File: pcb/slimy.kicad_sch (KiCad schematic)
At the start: 3 parts, among them U1 Teensy3.2, U2 PIM447

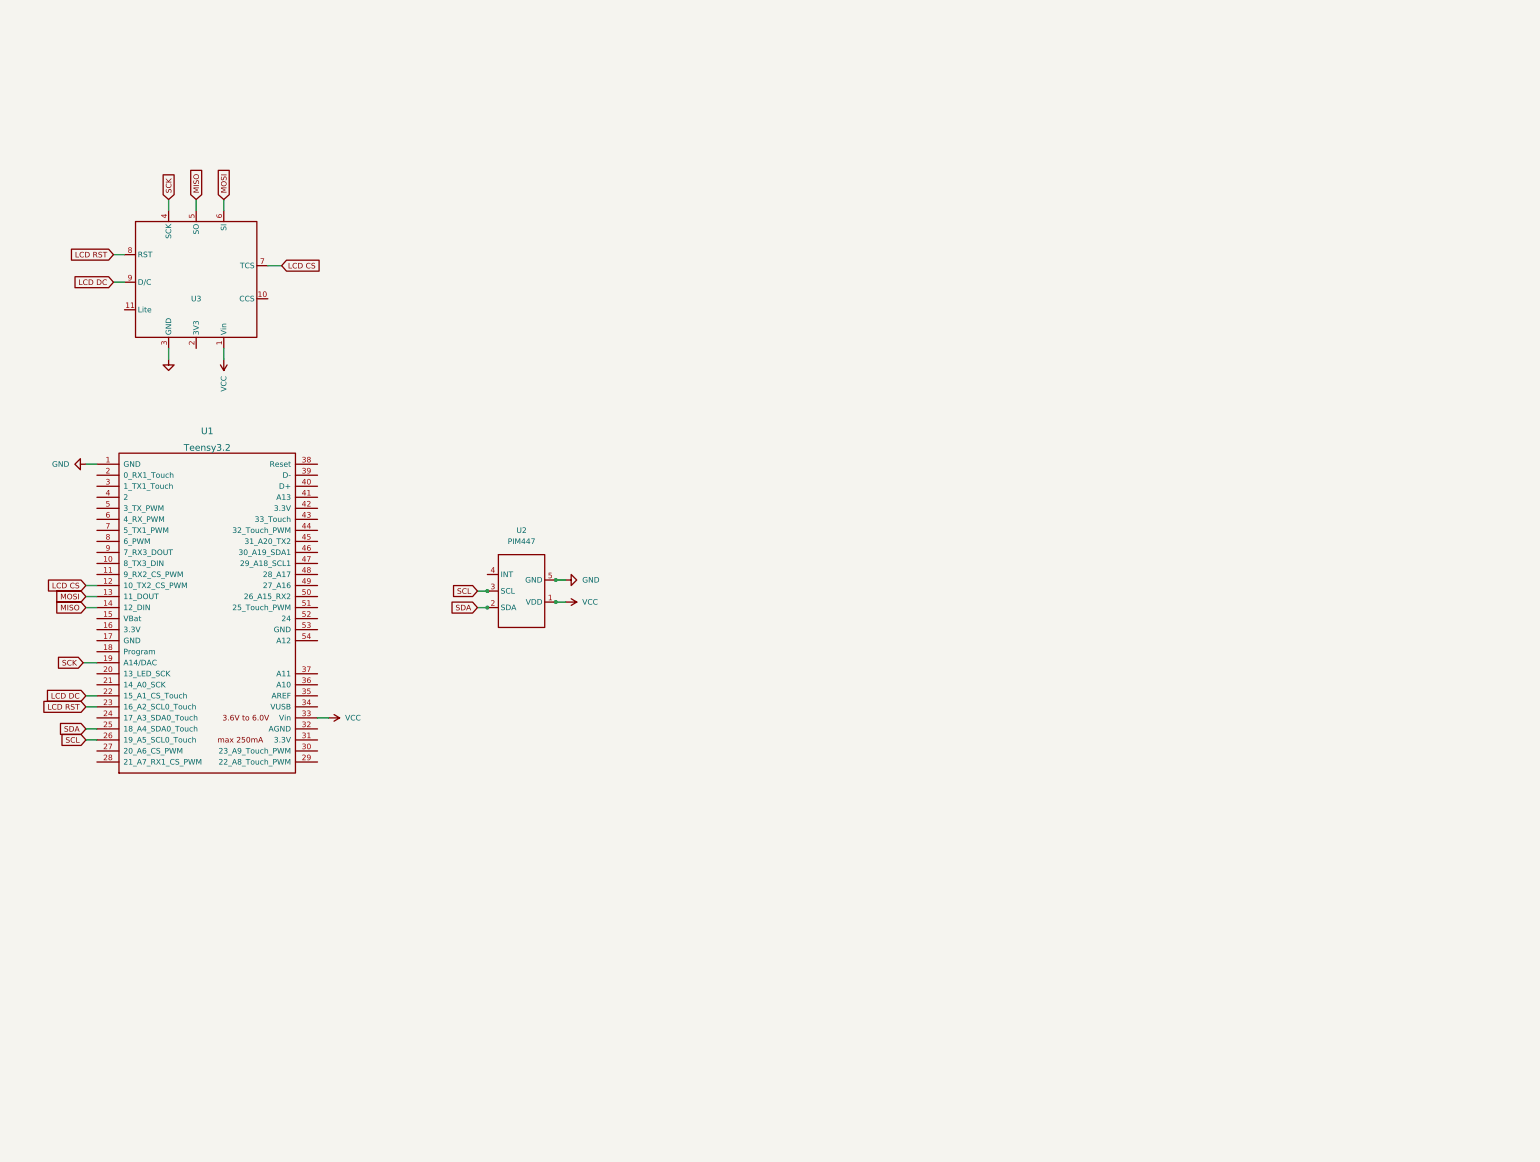
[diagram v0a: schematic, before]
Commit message: WIP keyboard pcb design
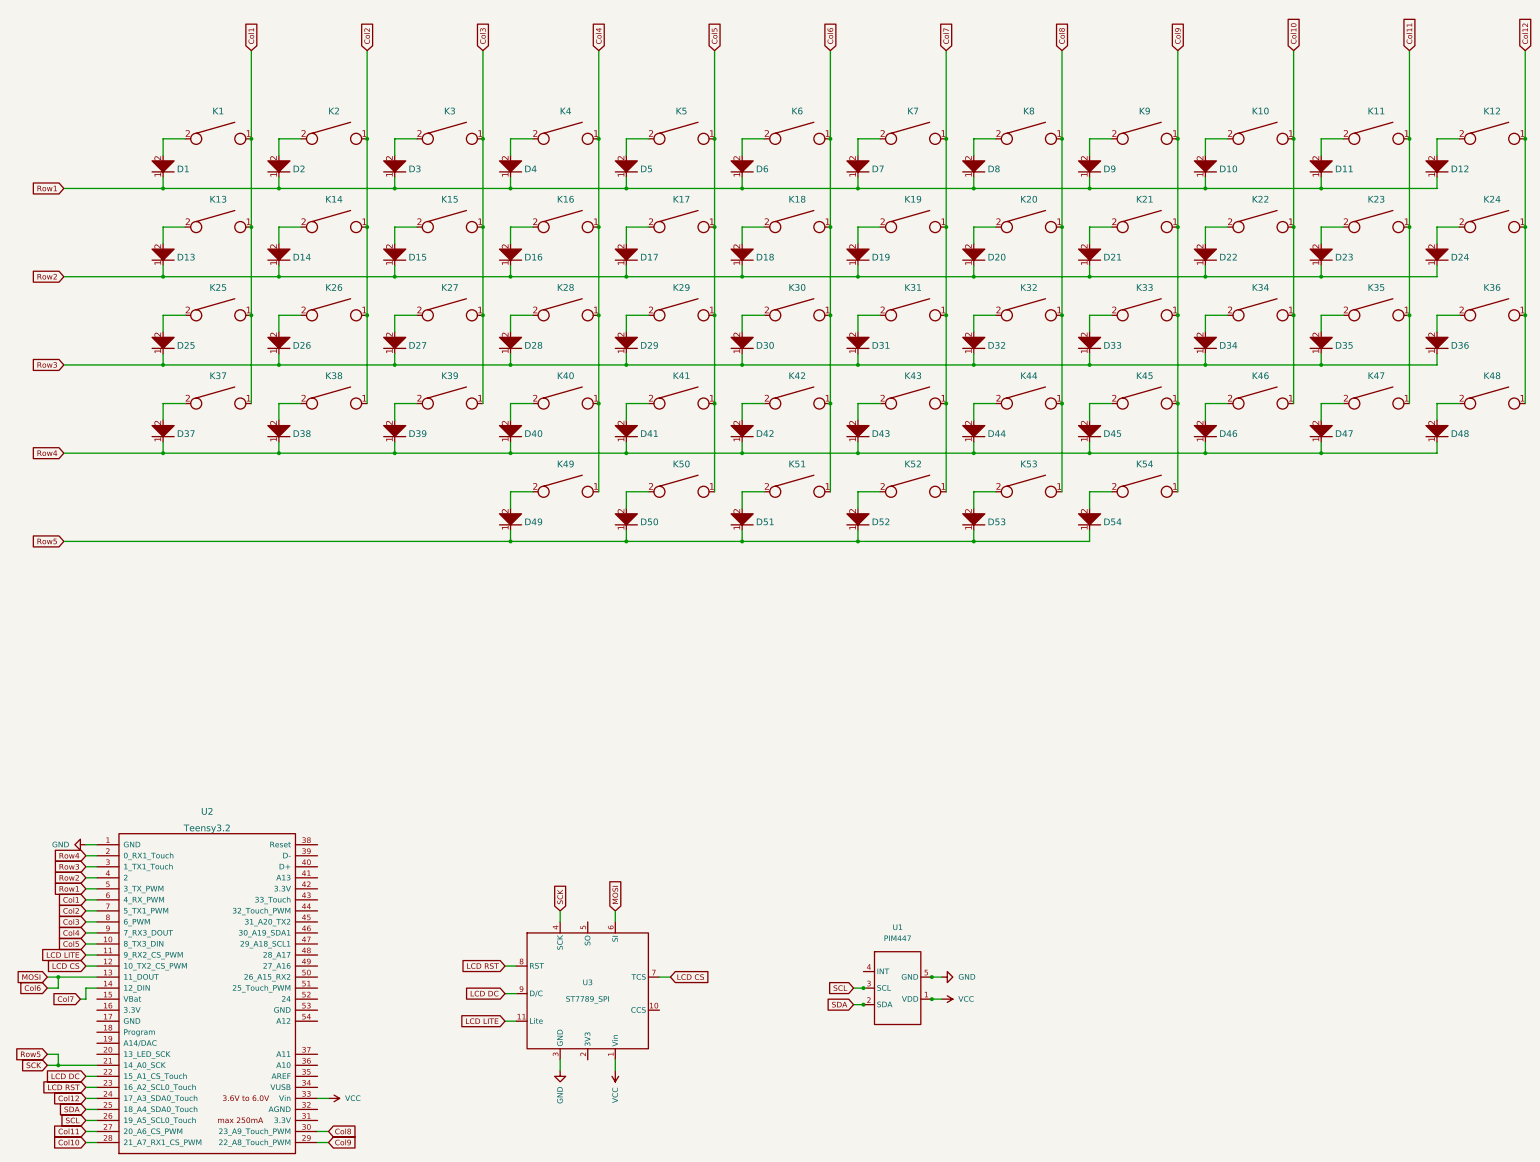
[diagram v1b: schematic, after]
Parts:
- removed U3: (no value), symbol my_lib:ST7789_240x240
- added D1, D10, D11, D12, D13, D14, D15, D16, D17, D18, D19, D2, D20, D21, D22, D23, D24, D25, D26, D27, D28, D29, D3, D30, D31, D32, D33, D34, D35, D36, D37, D38, D39, D4, D40, D41, D42, D43, D44, D45, D46, D47, D48, D49, D5, D50, D51, D52, D53, D54, D6, D7, D8, D9: D, my_lib:D_SOD123_axial, symbol kicad_lib_tmk:D
- added K1, K10, K11, K12, K13, K14, K15, K16, K17, K18, K19, K2, K20, K21, K22, K23, K24, K25, K26, K27, K28, K29, K3, K30, K31, K32, K33, K34, K35, K36, K37, K38, K39, K4, K40, K41, K42, K43, K44, K45, K46, K47, K48, K49, K5, K50, K51, K52, K53, K54, K6, K7, K8, K9: KEYSW, my_lib:MX-1U-Hotswap-Antishear, symbol kicad_lib_tmk:KEYSW
- added U3: ST7789_SPI, my_lib:ST7789_1.3_240x240, symbol my_lib:ST7789_SPI
- U1: renamed from U2; footprint (none) -> my_lib:PIM447
- U2: renamed from U1; footprint (none) -> teensy:Teensy30_31_32_All_Pins
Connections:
- net GND: now also U3.3 (GND)
- net LCD CS: now also U3.7 (TCS)
- net LCD DC: now also U3.9 (D/C)
- net LCD RST: now also U3.8 (RST)
- net VCC: now also U3.1 (Vin)
- net Col5: now reaches U2.10 (8_TX3_DIN)
- net Col5: now also K17.1, K29.1, K41.1, K5.1, K50.1
- net LCD LITE: now reaches U2.11 (9_RX2_CS_PWM)
- net LCD LITE: now also U3.11 (Lite)
- net Row4: now reaches U2.2 (0_RX1_Touch)
- net Row4: now also D37.1, D38.1, D39.1, D40.1, D41.1, D42.1, D43.1, D44.1, D45.1, D46.1, D47.1, D48.1
- net Row5: now reaches U2.21 (14_A0_SCK)
- net Row5: now also D49.1, D50.1, D51.1, D52.1, D53.1, D54.1, U3.4 (SCK)
- net Col12: now reaches U2.24 (17_A3_SDA0_Touch)
- net Col12: now also K12.1, K24.1, K36.1, K48.1
- net Col11: now reaches U2.27 (20_A6_CS_PWM)
- net Col11: now also K11.1, K23.1, K35.1, K47.1
- net Col10: now reaches U2.28 (21_A7_RX1_CS_PWM)
- net Col10: now also K10.1, K22.1, K34.1, K46.1
- net Col9: now reaches U2.29 (22_A8_Touch_PWM)
- net Col9: now also K21.1, K33.1, K45.1, K54.1, K9.1
- net Row3: now reaches U2.3 (1_TX1_Touch)
- net Row3: now also D25.1, D26.1, D27.1, D28.1, D29.1, D30.1, D31.1, D32.1, D33.1, D34.1, D35.1, D36.1
- net Col8: now reaches U2.30 (23_A9_Touch_PWM)
- net Col8: now also K20.1, K32.1, K44.1, K53.1, K8.1
- net Row2: now reaches U2.4 (2)
- net Row2: now also D13.1, D14.1, D15.1, D16.1, D17.1, D18.1, D19.1, D20.1, D21.1, D22.1, D23.1, D24.1
- net Row1: now reaches U2.5 (3_TX_PWM)
- net Row1: now also D1.1, D10.1, D11.1, D12.1, D2.1, D3.1, D4.1, D5.1, D6.1, D7.1, D8.1, D9.1
- net Col1: now reaches U2.6 (4_RX_PWM)
- net Col1: now also K1.1, K13.1, K25.1, K37.1
- net Col2: now reaches U2.7 (5_TX1_PWM)
- net Col2: now also K14.1, K2.1, K26.1, K38.1
- net Col3: now reaches U2.8 (6_PWM)
- net Col3: now also K15.1, K27.1, K3.1, K39.1
- net Col4: now reaches U2.9 (7_RX3_DOUT)
- net Col4: now also K16.1, K28.1, K4.1, K40.1, K49.1
- net MISO renamed Col7
- net Col7: now also K19.1, K31.1, K43.1, K52.1, K7.1
- net MOSI renamed Col6
- net Col6: now also K18.1, K30.1, K42.1, K51.1, K6.1, U3.6 (SI)
- net SCK: no longer names the net of U2.19 (A14/DAC)
- new net: D16.2, K16.2
- new net: D44.2, K44.2
- new net: D33.2, K33.2
- new net: D17.2, K17.2
- new net: D42.2, K42.2
- new net: D36.2, K36.2
- new net: D11.2, K11.2
- new net: D41.2, K41.2
- new net: D5.2, K5.2
- new net: D6.2, K6.2
- new net: D15.2, K15.2
- new net: D48.2, K48.2
- new net: D28.2, K28.2
- new net: D46.2, K46.2
- new net: D34.2, K34.2
- new net: D21.2, K21.2
- new net: D24.2, K24.2
- new net: D31.2, K31.2
- new net: D40.2, K40.2
- new net: D20.2, K20.2
- new net: D12.2, K12.2
- new net: D29.2, K29.2
- new net: D2.2, K2.2
- new net: D18.2, K18.2
- new net: D4.2, K4.2
- new net: D49.2, K49.2
- new net: D43.2, K43.2
- new net: D37.2, K37.2
- new net: D7.2, K7.2
- new net: D8.2, K8.2
- new net: D9.2, K9.2
- new net: D10.2, K10.2
- new net: D54.2, K54.2
- new net: D32.2, K32.2
- new net: D52.2, K52.2
- new net: D38.2, K38.2
- new net: D13.2, K13.2
- new net: D25.2, K25.2
- new net: D53.2, K53.2
- new net: D22.2, K22.2
- new net: D26.2, K26.2
- new net: D23.2, K23.2
- new net: D50.2, K50.2
- new net: D30.2, K30.2
- new net: D27.2, K27.2
- new net: D19.2, K19.2
- new net: D1.2, K1.2
- new net: D14.2, K14.2
- new net: D39.2, K39.2
- new net: D35.2, K35.2
- new net: D45.2, K45.2
- new net: D3.2, K3.2
- new net: D47.2, K47.2
- new net: D51.2, K51.2
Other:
- moved on the sheet: U1, U2

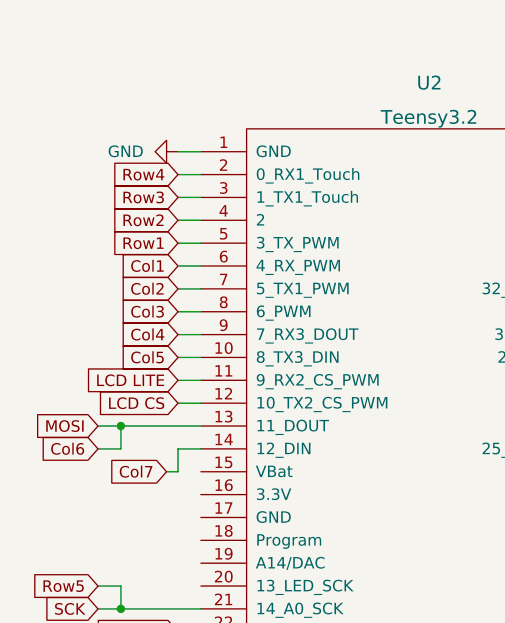
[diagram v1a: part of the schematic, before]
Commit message: First iteration design pt2
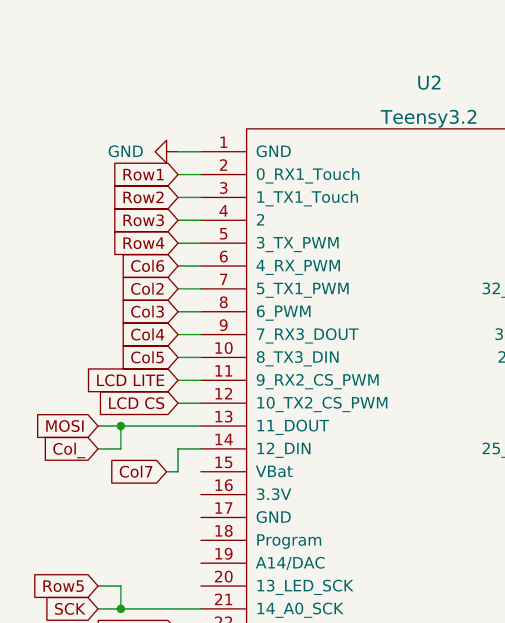
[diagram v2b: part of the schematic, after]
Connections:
- net Col1: no longer U2.6 (4_RX_PWM)
- net Col6: now also U2.6 (4_RX_PWM); no longer U2.13 (11_DOUT), U3.6 (SI)
- net Row1: now also U2.2 (0_RX1_Touch); no longer U2.5 (3_TX_PWM)
- net Row2: now also U2.3 (1_TX1_Touch); no longer U2.4 (2)
- net Row3: now also U2.4 (2); no longer U2.3 (1_TX1_Touch)
- net Row4: now also U2.5 (3_TX_PWM); no longer U2.2 (0_RX1_Touch)
- new net Col_: U2.13 (11_DOUT), U3.6 (SI)
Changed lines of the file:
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@@
     )
   )
-  (global_label "Row2" (shape input) (at 35.56 214.63 180) (fields_autoplaced)
+  (global_label "Row3" (shape input) (at 35.56 214.63 180) (fields_autoplaced)
     (effects (font (size 1.27 1.27)) (justify right))
     (property "Intersheet References" "${INTERSHEET_REFS}" (id 0) (at 28.1879 214.5506 0)
@@
     )
   )
-  (global_label "Row1" (shape input) (at 35.56 217.17 180) (fields_autoplaced)
+  (global_label "Row4" (shape input) (at 35.56 217.17 180) (fields_autoplaced)
     (effects (font (size 1.27 1.27)) (justify right))
     (property "Intersheet References" "${INTERSHEET_REFS}" (id 0) (at 28.1879 217.0906 0)
@@
     )
   )
-  (global_label "Row3" (shape input) (at 35.56 212.09 180) (fields_autoplaced)
+  (global_label "Row2" (shape input) (at 35.56 212.09 180) (fields_autoplaced)
     (effects (font (size 1.27 1.27)) (justify right))
     (property "Intersheet References" "${INTERSHEET_REFS}" (id 0) (at 28.1879 212.0106 0)
@@
     )
   )
-  (global_label "Col6" (shape input) (at 26.67 240.03 180) (fields_autoplaced)
-    (effects (font (size 1.27 1.27)) (justify right))
-    (property "Intersheet References" "${INTERSHEET_REFS}" (id 0) (at 19.9631 240.1094 0)
+  (global_label "Col_" (shape input) (at 26.67 240.03 180) (fields_autoplaced)
+    (effects (font (size 1.27 1.27)) (justify right))
+    (property "Intersheet References" "${INTERSHEET_REFS}" (id 0) (at 20.205 239.9506 0)
       (effects (font (size 1.27 1.27)) (justify right) hide)
     )
@@
     )
   )
-  (global_label "Col1" (shape input) (at 35.56 219.71 180) (fields_autoplaced)
+  (global_label "Col6" (shape input) (at 35.56 219.71 180) (fields_autoplaced)
     (effects (font (size 1.27 1.27)) (justify right))
     (property "Intersheet References" "${INTERSHEET_REFS}" (id 0) (at 28.8531 219.6306 0)
@@
     )
   )
-  (global_label "Row4" (shape input) (at 35.56 209.55 180) (fields_autoplaced)
+  (global_label "Row1" (shape input) (at 35.56 209.55 180) (fields_autoplaced)
     (effects (font (size 1.27 1.27)) (justify right))
     (property "Intersheet References" "${INTERSHEET_REFS}" (id 0) (at 28.1879 209.4706 0)
